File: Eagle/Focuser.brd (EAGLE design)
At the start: 97.8 x 46.7 mm, 28 parts, among them IC1 L7805, IC2 L7805, Q1 IRF540, Q2 IRF540, Q3 IRF540

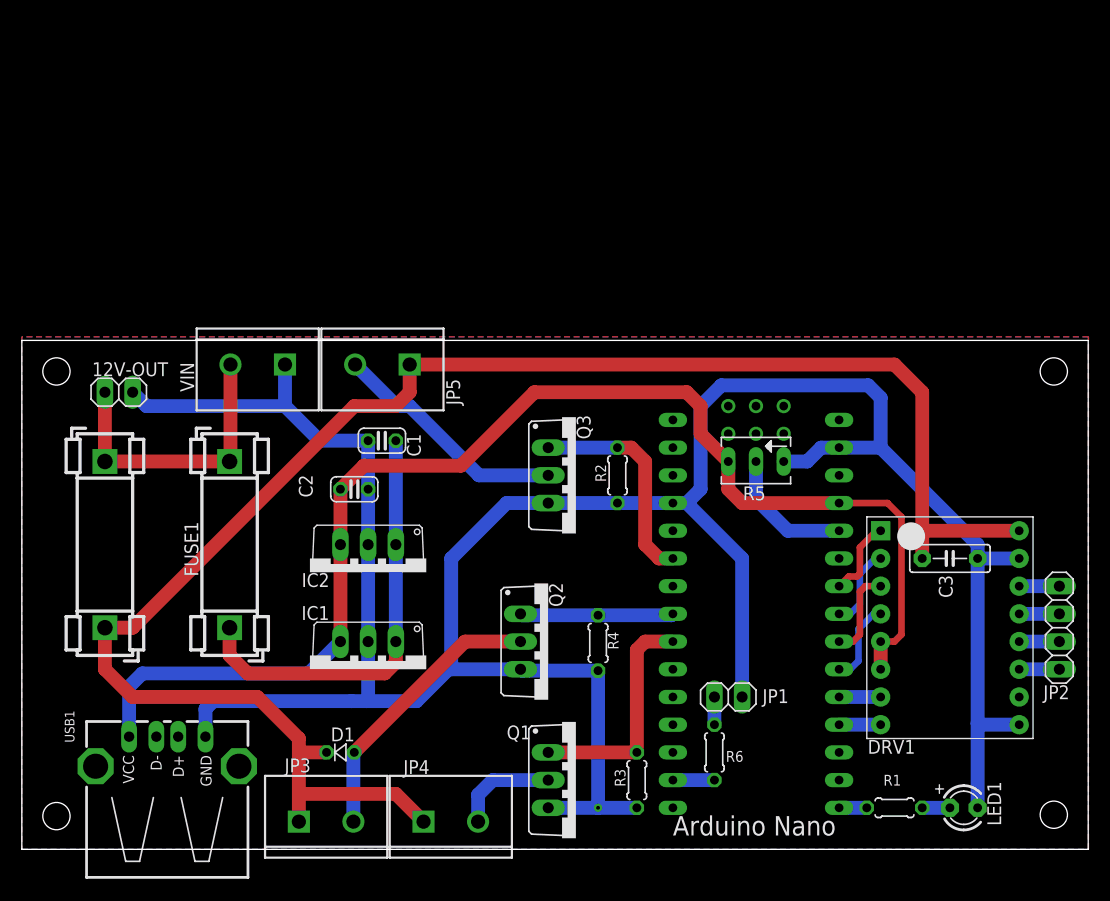
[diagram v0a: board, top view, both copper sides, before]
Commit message: Circuit for commercial version
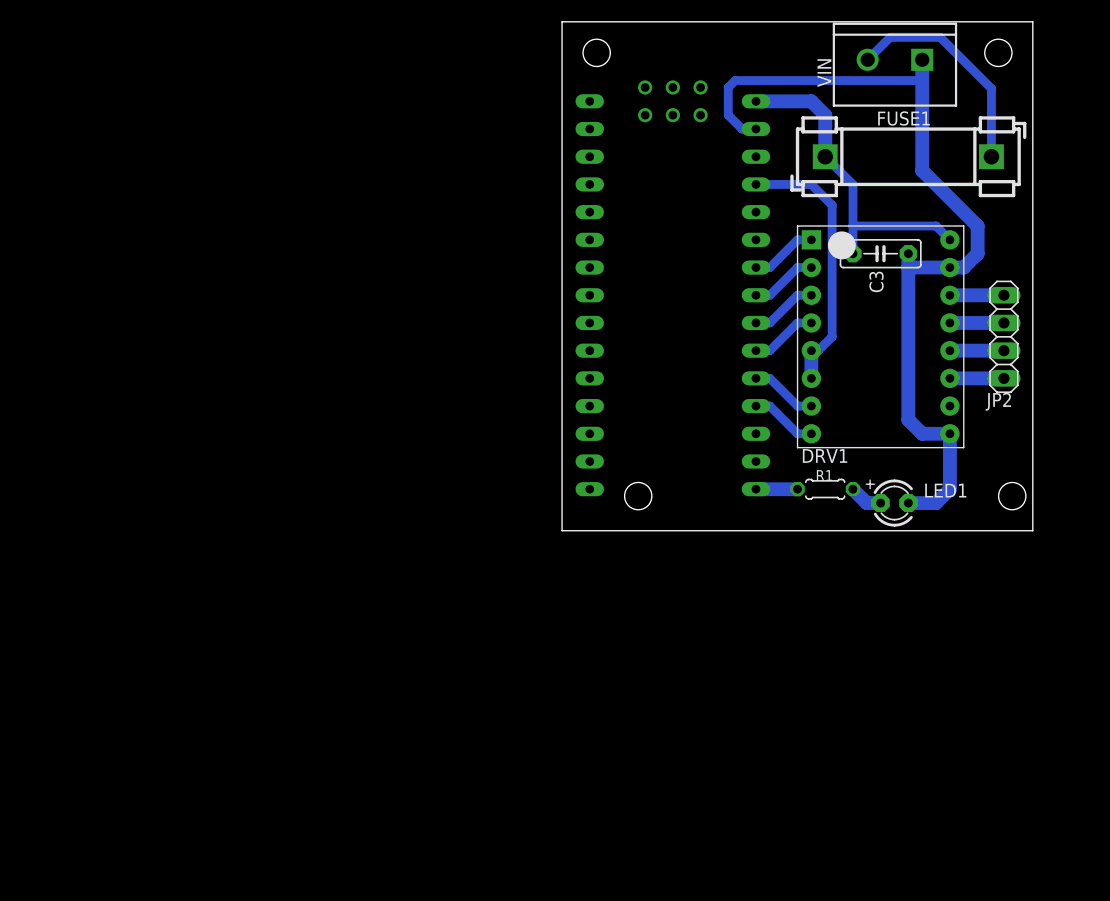
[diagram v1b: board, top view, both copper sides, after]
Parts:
- removed 12V-OUT, JP1: (no value), pinhead:1X02
- removed C1, C2: 10uF, rcl:C025-024X044
- removed D1: (no value), diode:D-2.5
- removed FUSE2: 2A, fuse:FUSE_HOLDER_5X20MM
- removed IC1, IC2: L7805, linear:TO220V
- removed JP3, JP4, JP5: (no value), SparkFun-Connectors:SCREWTERMINAL-5MM-2
- removed Q1, Q2, Q3: IRF540, transistor-power:TO220BV
- removed R2, R3, R4: 4.7K, rcl:0204/5
- removed R5: (no value), pot:B64Y
- removed R6: 220R, resistor:0204/5
- removed USB1: FEMALE A, Seeed-Connector:USB4+2P-2.0-90D
- FUSE1: value 1.5A -> 1A
- moved FUSE1 75.2 mm to (39.4, 34.3), turned to 180 degrees
- moved VIN 64.8 mm to (33.0, 43.2)
- moved U$1 30.2 mm to (7.62, 30.5)
- moved R1 29.9 mm to (24.1, 3.81)
- moved C3 28.7 mm to (29.2, 25.4)
- moved LED1 28.7 mm to (30.5, 2.54)
- moved DRV1 27.4 mm to (21.6, 27.9)
- moved JP2 27.1 mm to (40.5, 17.8)
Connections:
- removed net D3: Q3.G, R2.2, U$1.D3
- removed net D5: Q2.G, R4.2, U$1.D5
- removed net D6: Q1.G, R3.2, U$1.D6
- removed net N$10: JP4.2, Q1.D
- removed net N$11: JP5.2, Q3.D
- removed net N$19: JP1.1, R6.1
- removed net N$2: R5.S, U$1.A7
- removed net N$3: R6.2, U$1.D11
- removed net N$4: C1.1, FUSE1.2, IC1.1, IC2.1
- removed net N$8: 12V-OUT.2, FUSE1.1, FUSE2.1, VIN.2
- removed net N$9: D1.A, JP3.2, Q2.D
- new net N$7: FUSE1.1, VIN.2
- net +12V: now also FUSE1.2, U$1.RAW; no longer D1.C, FUSE2.2, JP3.1, JP4.1, JP5.1
- net +5V: no longer C2.1, IC1.3, IC2.3, R5.A, USB1.1
- net GND: no longer 12V-OUT.1, C1.2, C2.2, IC1.2, IC2.2, JP1.2, Q1.S, Q2.S, Q3.S, R2.1, R3.1, R4.1, R5.E, U$1.GND1, USB1.4
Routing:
- net GND: track 251.4 -> 79.4 mm, vias 1 -> 0
- net +12V: track 158.6 -> 30.0 mm
- net +5V: track 118.0 -> 24.8 mm
- net N$4: track 39.2 -> 0.00 mm
- net N$8: track 26.7 -> 0.00 mm
- net N$9: track 25.8 -> 0.00 mm
- net N$11: track 21.9 -> 0.00 mm
- net D6: track 21.1 -> 0.00 mm
- net N$7: track 0.00 -> 20.4 mm
- net D3: track 20.1 -> 0.00 mm
- net D5: track 14.1 -> 0.00 mm
- net N$2: track 12.3 -> 0.00 mm
- net N$10: track 9.45 -> 0.00 mm
- net N$3: track 3.81 -> 0.00 mm
- net N$18: track 8.73 -> 6.13 mm
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- removed copper zone on layer 1, net GND
- removed copper zone on layer 16, net GND
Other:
- board size 97.8 x 46.7 mm -> 43.2 x 46.7 mm
- board text removed: "Arduino Nano"
